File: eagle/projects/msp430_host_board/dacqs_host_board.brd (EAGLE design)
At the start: 127 x 102 mm, 181 parts, among them J1 MOL-SL-4-RA, J10 MOL-SL-3-V, J13 JST-PH-2TH-RA, J14 USB_MICROB_RECPT, J16 MOL-SL-2-RA, J17 CLM-112-02-L-D-IMU-MOUNT_IMU, J18 MOLSL-7-RA, J2 MOL-SL-4-RA, J3 MOL-SL-4-RA, J4 MOL-SL-4-RA, J5 MOL-SL-5-RA, J6 MOL-SL-3-V, J7 MOL-SL-5-V, J8 MOL-SL-3-RA, J9 MOL-SL-4-RA, U1 MSP430FR4994, U10 LSM9DS1, U2 MSP430FR4994, U3 PCT2075D,118, U4 MS560702BA03-50, U5 TPS61240DRVR, U6 LP5907_DBV_5, U7 MCP73831T, U8 INA219AIDCNR, Y1 32.768kHz, Y3 32.768kHz

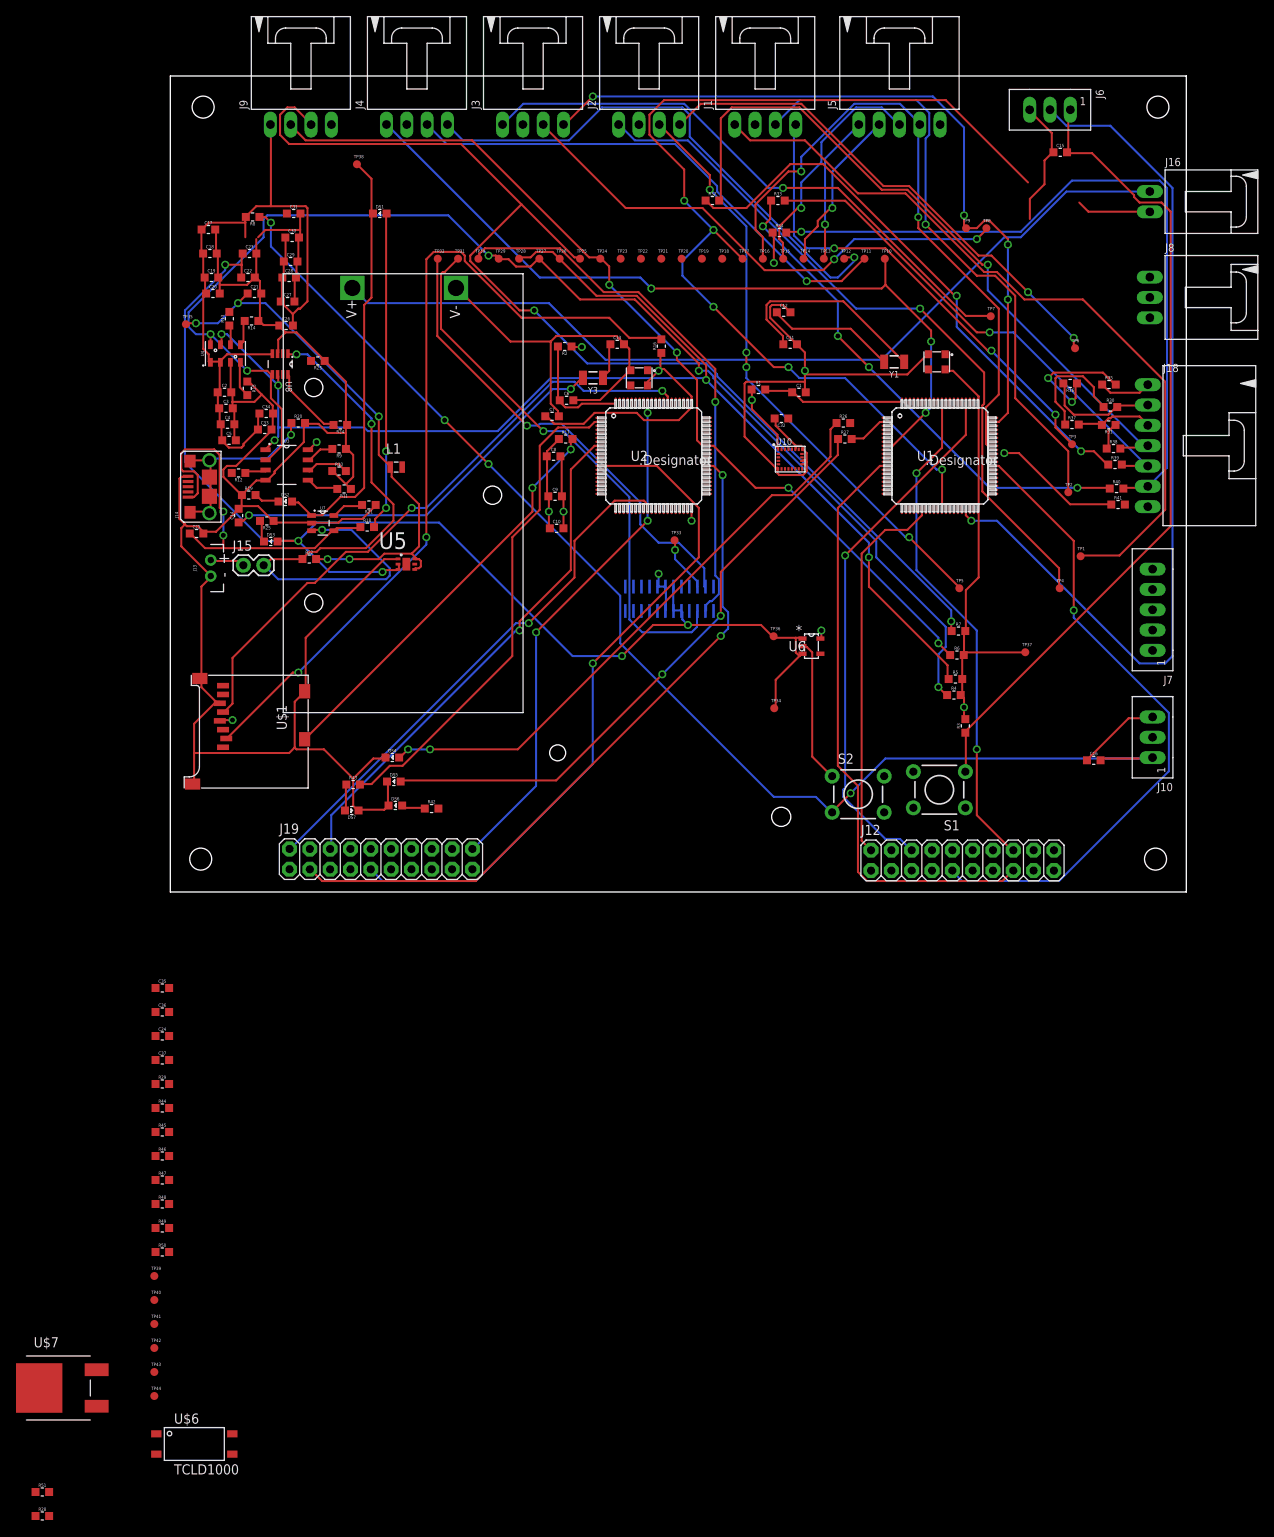
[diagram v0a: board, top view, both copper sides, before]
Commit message: Started power layout
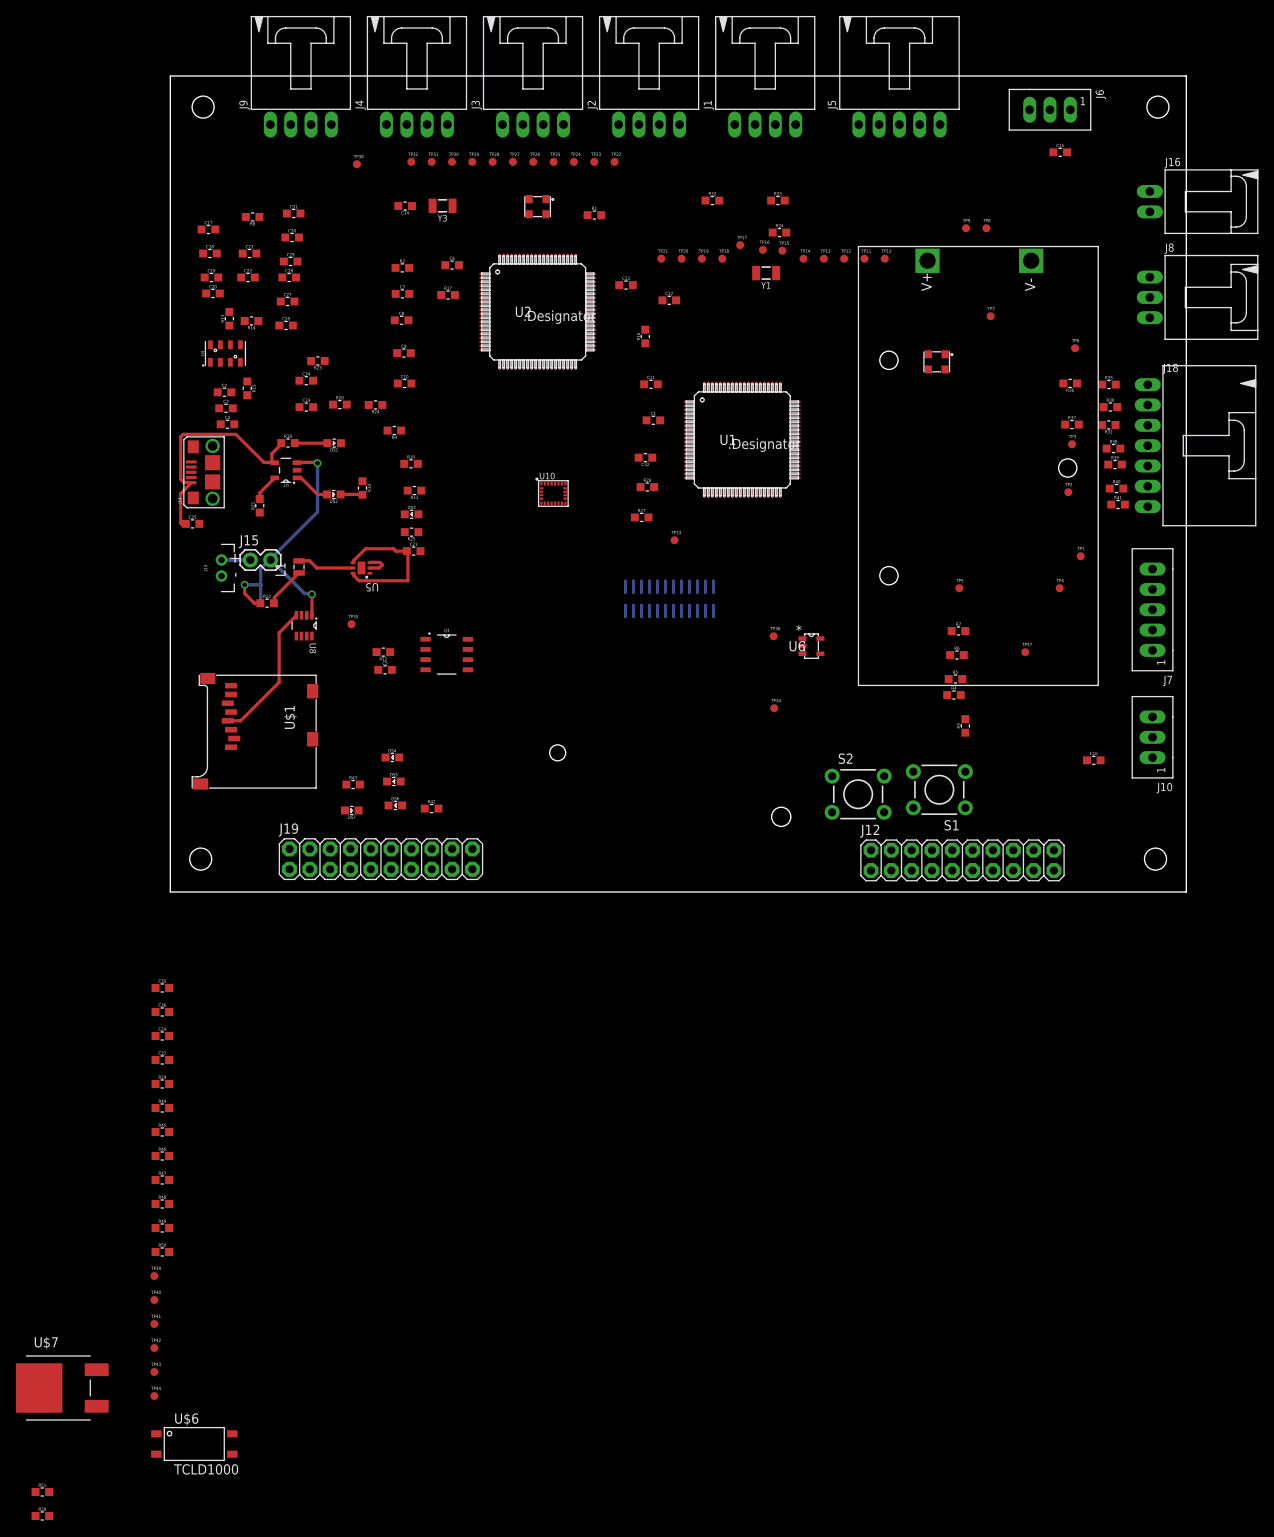
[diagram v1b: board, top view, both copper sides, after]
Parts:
- moved BAT1 72.0 mm to (116.0, 25.8)
- moved C14 43.9 mm to (29.4, 85.7), turned to 180 degrees
- moved TP35 42.8 mm to (22.6, 33.5)
- moved C21 37.9 mm to (30.4, 42.6)
- moved C5 34.7 mm to (26.8, 27.8)
- moved U8 32.8 mm to (16.7, 33.3)
- moved U3 31.0 mm to (34.5, 29.7)
- moved R1 29.9 mm to (53.0, 84.6)
- moved U10 29.9 mm to (47.9, 49.8)
- moved DS1 29.3 mm to (20.5, 56.1), turned to 180 degrees
- moved R12 28.8 mm to (26.6, 30.0)
- moved Y3 28.6 mm to (34.0, 85.8)
- moved R27 27.2 mm to (58.9, 46.8)
- moved C10 26.2 mm to (29.3, 63.6)
- moved C9 26.0 mm to (29.2, 67.4)
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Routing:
- net GND: track 444.7 -> 0.00 mm, vias 3 -> 0
- net +3V3: track 211.4 -> 17.7 mm, vias 9 -> 0
- net SENSE_SCL_1: track 162.8 -> 0.00 mm, vias 5 -> 0
- net SENSE_SDA_1: track 159.1 -> 0.00 mm, vias 5 -> 0
- net RST_SBWTDIO_MOTOR: track 157.0 -> 0.00 mm, vias 4 -> 0
- net +5V: track 158.0 -> 3.42 mm, vias 5 -> 0
- net SENSE_SCL_2: track 142.4 -> 0.00 mm, vias 2 -> 0
- net CUTDOWN_EN: track 129.7 -> 0.00 mm, vias 5 -> 0
- net SENSE_SDA_2: track 116.7 -> 0.00 mm, vias 4 -> 0
- net SBWTCK_HOST: track 112.5 -> 0.00 mm, vias 1 -> 0
- net VBAT_POS: track 112.1 -> 0.00 mm
- net SD_CS: track 105.4 -> 0.00 mm, vias 2 -> 0
- net RST_SBWTDIO_HOST: track 102.2 -> 0.00 mm
- net UART_4_TX: track 99.6 -> 0.00 mm, vias 3 -> 0
- net RST_PI_3: track 96.3 -> 0.00 mm, vias 4 -> 0
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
